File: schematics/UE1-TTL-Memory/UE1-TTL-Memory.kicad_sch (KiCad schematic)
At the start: 6 parts, among them J1 Edge 1, J2 Edge 2

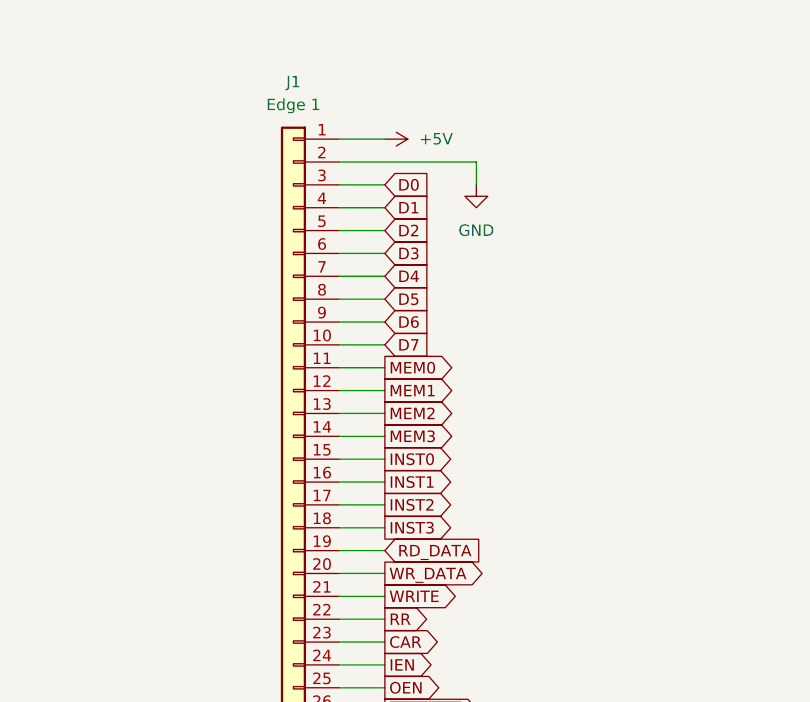
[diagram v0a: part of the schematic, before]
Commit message: Lay out memory board
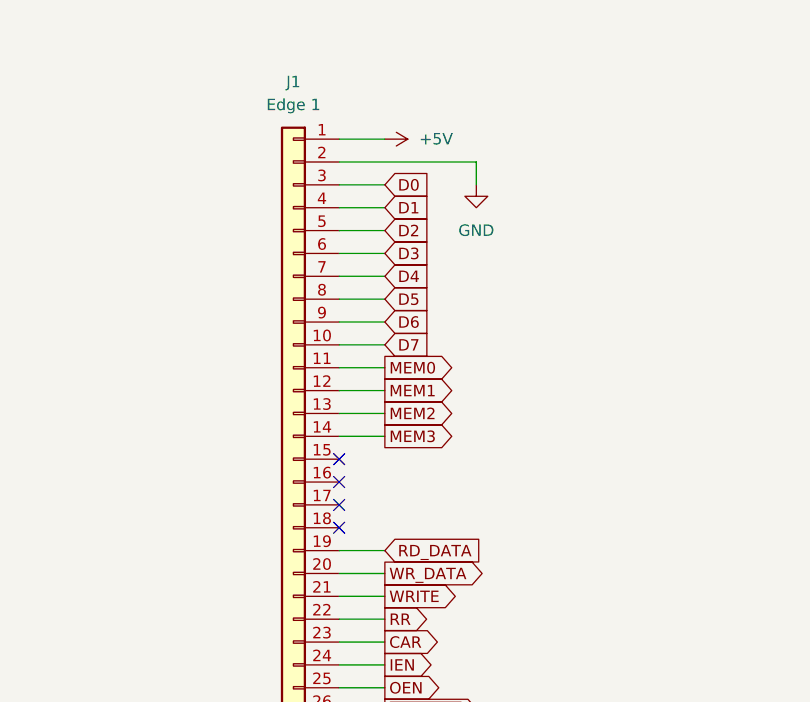
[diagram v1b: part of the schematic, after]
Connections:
- net INST0: no longer names the net of J1.15 (Pin_15)
- net INST1: no longer names the net of J1.16 (Pin_16)
- net INST2: no longer names the net of J1.17 (Pin_17)
- net INST3: no longer names the net of J1.18 (Pin_18)
- no-connect marks 1 -> 5
